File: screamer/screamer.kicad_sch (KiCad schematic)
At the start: 6 parts

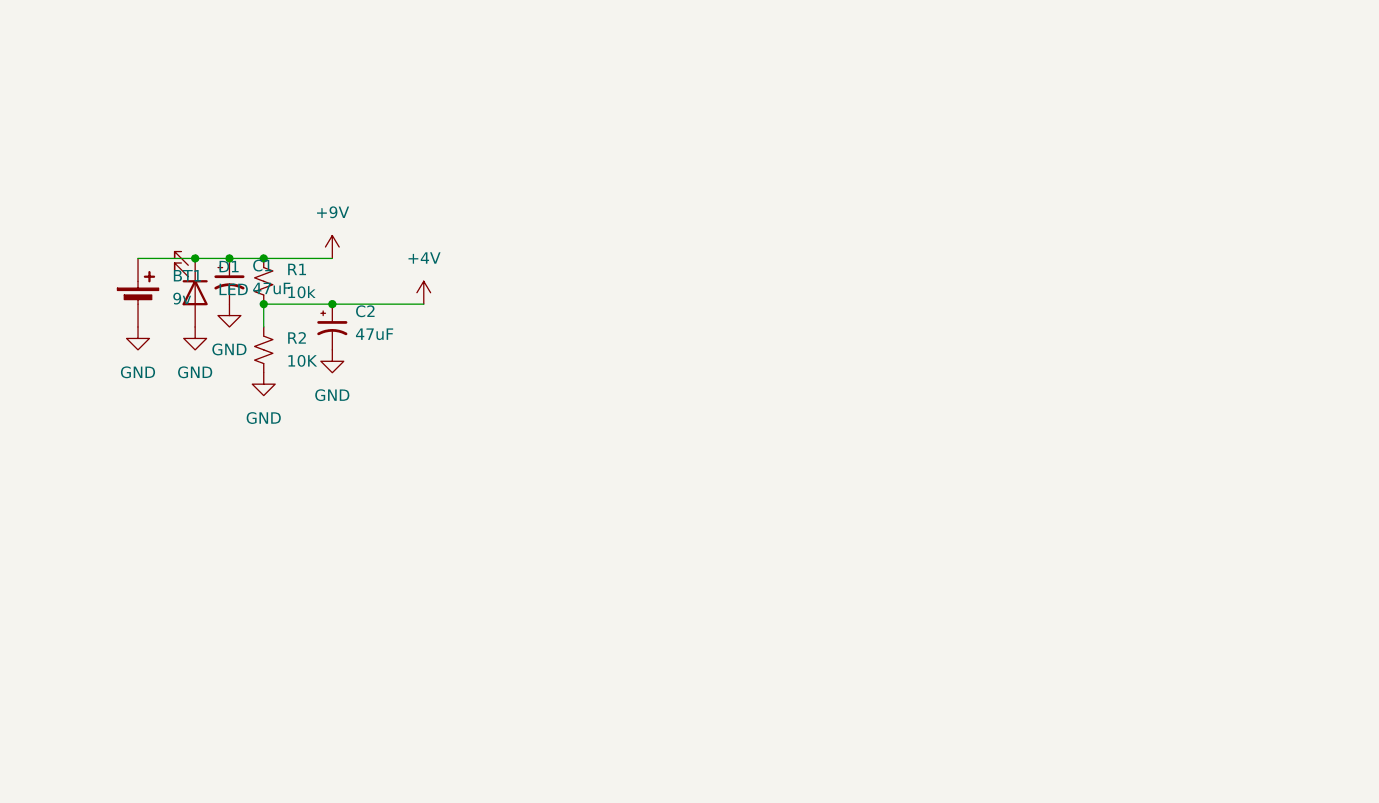
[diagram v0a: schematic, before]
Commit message: Finished circuit
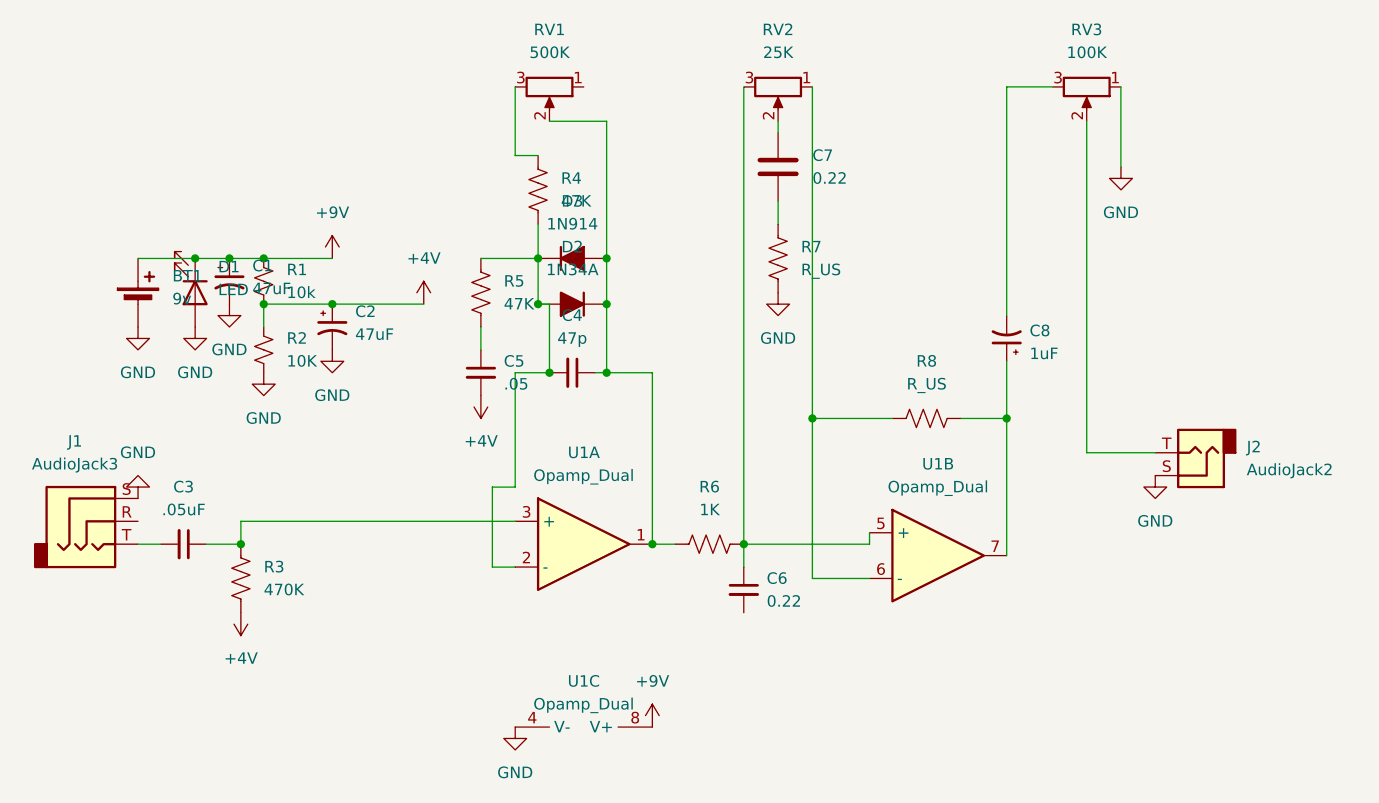
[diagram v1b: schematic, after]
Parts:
- added C3: .05uF, symbol Device:C_Small
- added C4: 47p, symbol Device:C_Small
- added C5: .05, symbol Device:C_Small
- added C6: 0.22, symbol Device:C_Small
- added C7: 0.22, symbol Device:C
- added C8: 1uF, symbol Device:C_Polarized_Small_US
- added D2: 1N34A, symbol Device:D_Filled
- added D3: 1N914, symbol Device:D_Filled
- added J1: AudioJack3, symbol Connector_Audio:AudioJack3
- added J2: AudioJack2, symbol Connector_Audio:AudioJack2
- added R3: 470K, symbol Device:R_US
- added R4, R5: 47K, symbol Device:R_US
- added R6: 1K, symbol Device:R_US
- added R7, R8: R_US, symbol Device:R_US
- added RV1: 500K, symbol Device:R_Potentiometer
- added RV2: 25K, symbol Device:R_Potentiometer
- added RV3: 100K, symbol Device:R_Potentiometer
- added U1: Opamp_Dual, symbol Device:Opamp_Dual
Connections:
- net +4V: now also C5.2, R3.2
- net +9V: now also U1.8 (V+)
- net GND: now also J1.S, J2.S, R7.2, RV3.1, U1.4 (V-)
- new net: C7.2, R7.1
- new net: C4.1, D2.1 (K), D3.2 (A), R6.1, RV1.2, U1.1
- new net: C4.2, D2.2 (A), D3.1 (K), R4.2, R5.1, U1.2 (-)
- new net: C3.1, R3.1, U1.3 (+)
- new net: C5.1, R5.2
- new net: C3.2, J1.T
- new net: C8.1, R8.1, U1.7
- new net: C8.2, RV3.3
- new net: R4.1, RV1.3
- new net: C6.1, R6.2, RV2.3, U1.5 (+)
- new net: J2.T, RV3.2
- new net: R8.2, RV2.1, U1.6 (-)
- new net: C7.1, RV2.2

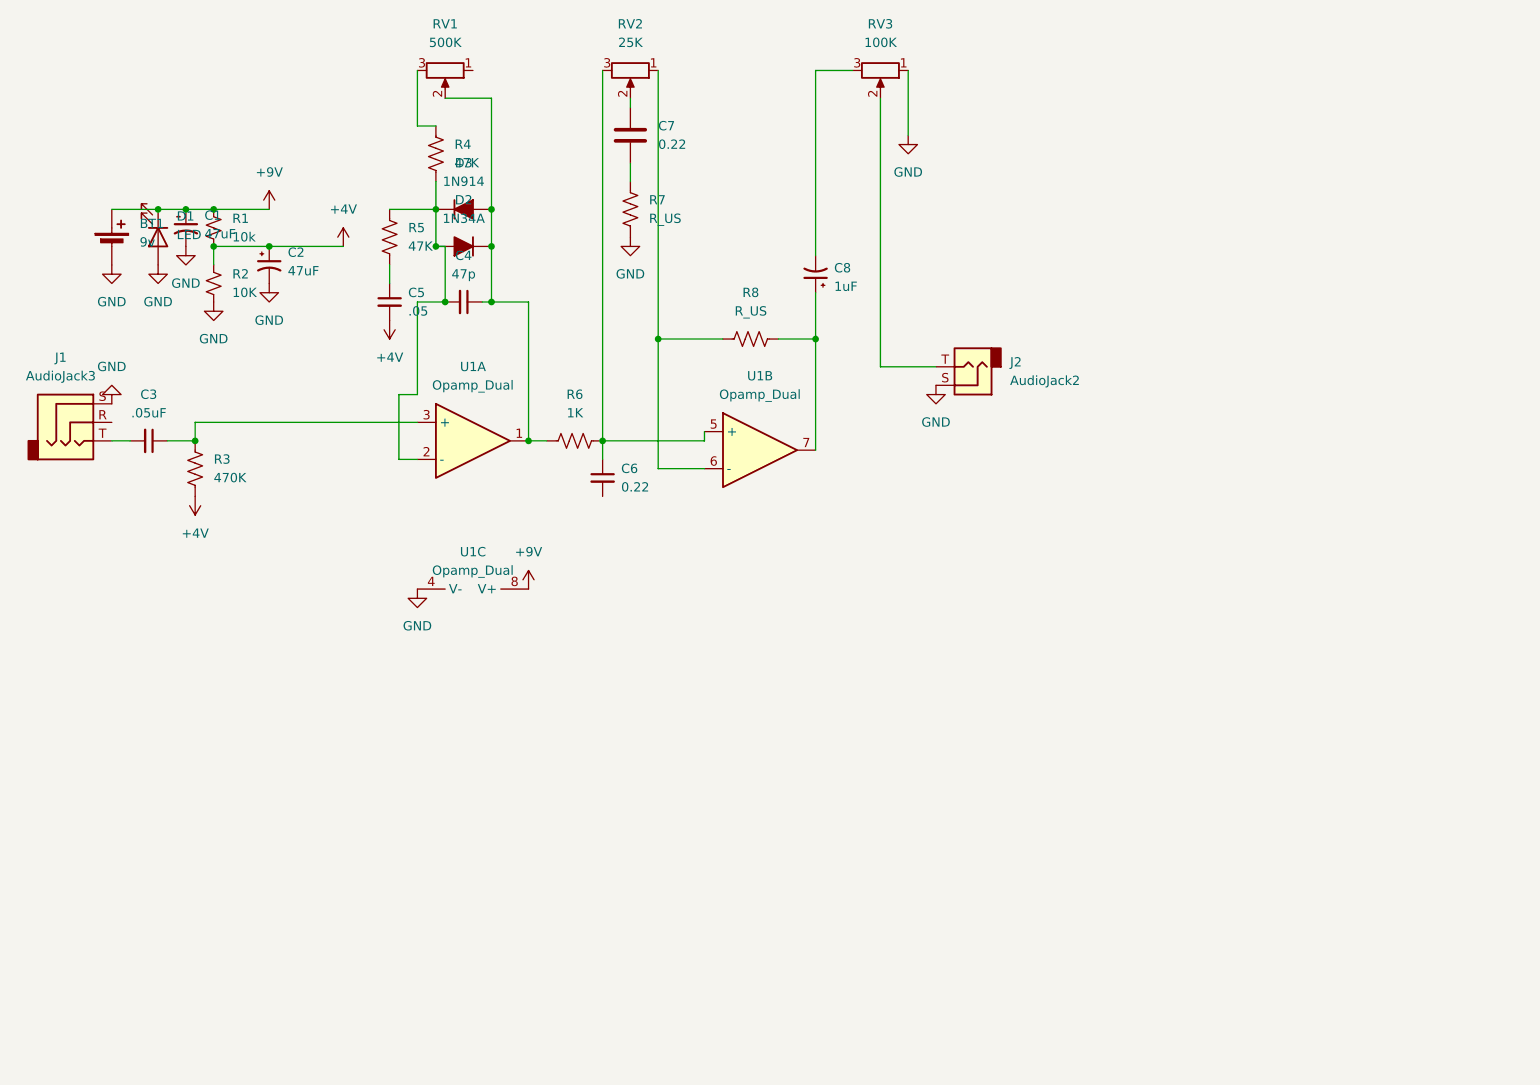
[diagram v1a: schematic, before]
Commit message: bunchastuff
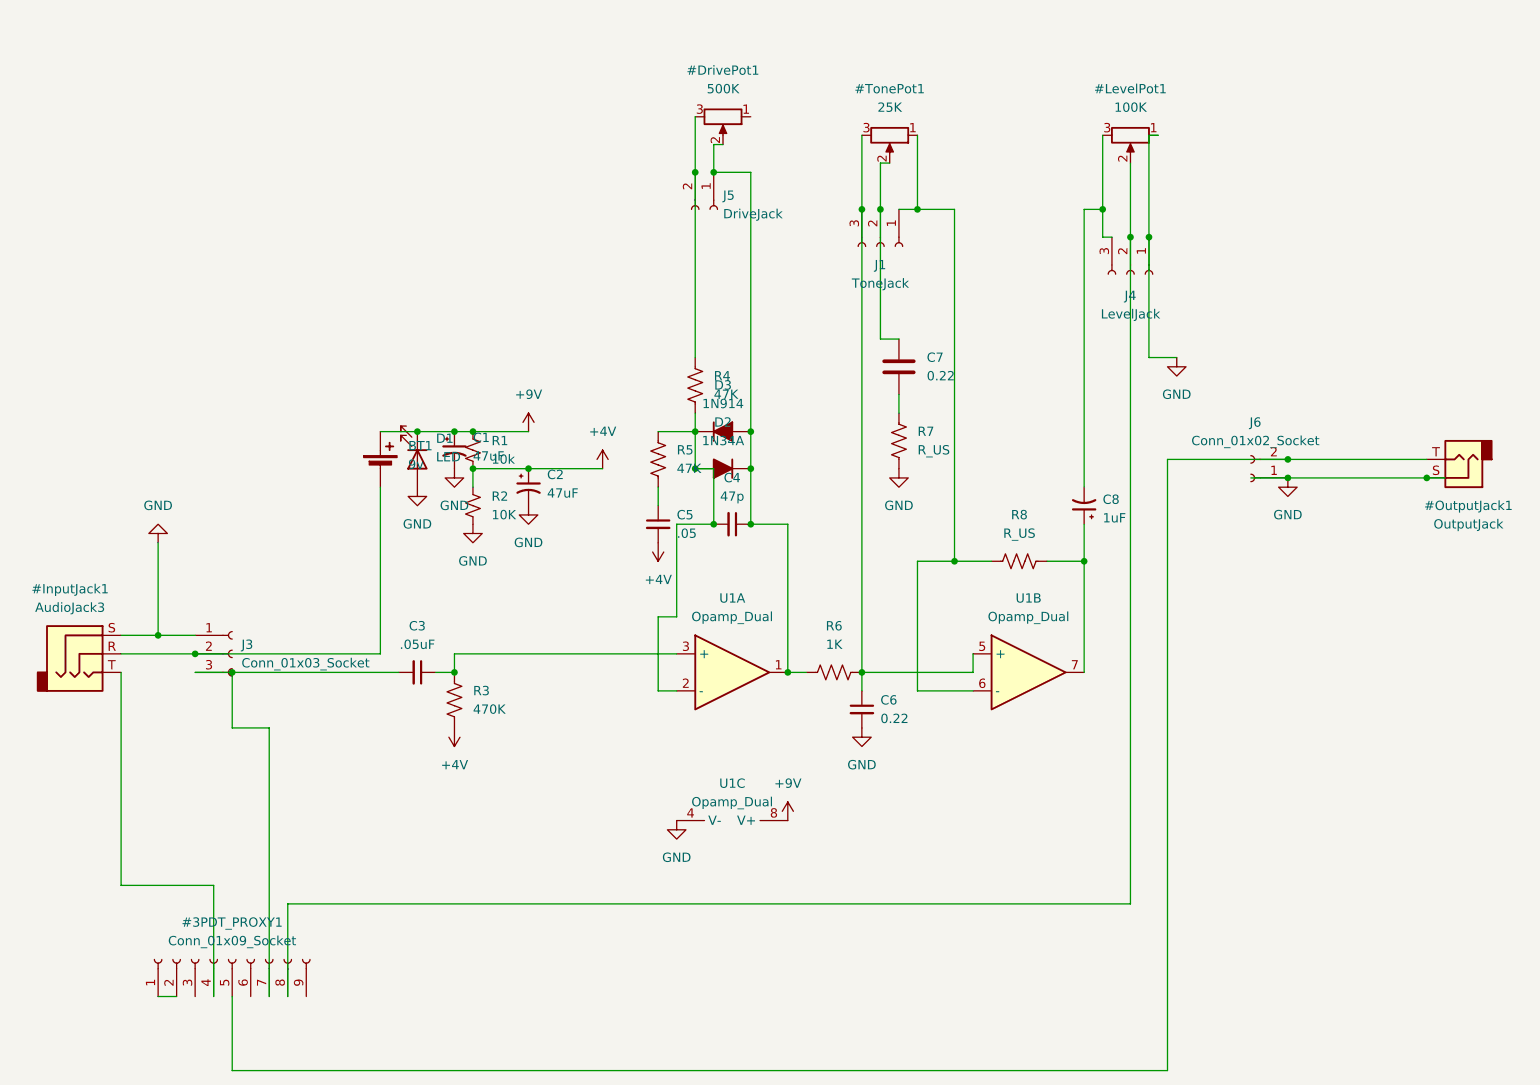
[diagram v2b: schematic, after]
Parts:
- added #3PDT_PROXY1: Conn_01x09_Socket, symbol Connector:Conn_01x09_Socket
- added J1: ToneJack, symbol Connector:Conn_01x03_Socket
- added J3: Conn_01x03_Socket, Connector:FanPinHeader_1x03_P2.54mm_Vertical, symbol Connector:Conn_01x03_Socket
- added J4: LevelJack, symbol Connector:Conn_01x03_Socket
- added J5: DriveJack, symbol Connector:Conn_01x02_Socket
- added J6: Conn_01x02_Socket, symbol Connector:Conn_01x02_Socket
- #OutputJack1: renamed from J2; value AudioJack2 -> OutputJack
- renumbered RV1 to #DrivePot1, J1 to #InputJack1, RV3 to #LevelPot1, RV2 to #TonePot1
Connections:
- net GND: now also C6.2, J3.1 (Pin_1), J4.1 (Pin_1), J6.1 (Pin_1); no longer BT1.2 (-)
- net at #DrivePot1.2, C4.1, D2.1 (K)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: now also J5.1 (Pin_1)
- net at C3.2: now also #3PDT_PROXY1.7 (Pin_7), J3.3 (Pin_3); no longer #InputJack1.T
- net at #LevelPot1.3, C8.2: now also J4.3 (Pin_3)
- net at #DrivePot1.3, R4.1: now also J5.2 (Pin_2)
- net at #TonePot1.3, C6.1, R6.2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: now also J1.3 (Pin_3)
- net at #InputJack1.R: now also BT1.2 (-), J3.2 (Pin_2)
- net at #OutputJack1.T: now also #3PDT_PROXY1.5 (Pin_5), J6.2 (Pin_2); no longer #LevelPot1.2
- net at #TonePot1.1, R8.2, U1.6 (-): now also J1.1 (Pin_1)
- net at #TonePot1.2, C7.1: now also J1.2 (Pin_2)
- new net: #3PDT_PROXY1.4 (Pin_4), #InputJack1.T
- new net: #3PDT_PROXY1.8 (Pin_8), #LevelPot1.2, J4.2 (Pin_2)
- new net: #3PDT_PROXY1.1 (Pin_1), #3PDT_PROXY1.2 (Pin_2)
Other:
- moved on the sheet: BT1, C1, C2, C3, C4, C5, C6, C7, C8, D1, D2, D3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
